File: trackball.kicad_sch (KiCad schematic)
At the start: 198 parts, among them J1 ZX-PM2.0-2-4PY, Q1 SI2302_C2891732, SW1 HX TC-5608-Y, SW2 HX TC-5608-Y, SW3 HX TC-5608-Y, SW4 HX TC-5608-Y, SW5 HX TC-5608-Y, SW6 HX TC-5608-Y, SW7 HX TC-5608-Y, SW8 HX TC-5608-Y, U1 SY8089A1AAC, U10 WS2812B, U11 WS2812B, U12 WS2812B, U13 WS2812B, U14 WS2812B, U15 WS2812B, U16 WS2812B, U17 WS2812B, U18 WS2812B, U19 WS2812B, U2 USB-TYPE-C-017, U20 WS2812B, U21 ANT3216LL00R2400A, U3 PMW3610, U4 PMW3610, U5 WS2812B, U6 WS2812B, U7 WS2812B, U8 WS2812B, U9 WS2812B, X1 XL7EL89CKI-111YLC-32M

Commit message: feat: rev.02 hardware
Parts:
- removed BAT1: ZX-SH1.0-3PLT, easyeda2kicad:CONN-SMD_3P-P1.00_HDGC_HDGC1002WV-S-3P, symbol easyeda2kicad:ZX-SH1.0-3PLT
- removed C1: CL05A106MP5NUNC_C315248, easyeda2kicad:C0402, symbol easyeda2kicad:CL05A106MP5NUNC_C315248
- removed C13, C14, C15, C17, C18, C19, C20, C24, C25, C28, C32, C33, C37, C38, C42, C46, C48, C49, C54, C55, C57: TCC0402X7R103M500AT, easyeda2kicad:C0402, symbol easyeda2kicad:TCC0402X7R103M500AT
- removed C16, C21, C22, C23, C30, C36, C43, C45, C51, C52: CC0402KRX7R7BB104, easyeda2kicad:C0402, symbol easyeda2kicad:CC0402KRX7R7BB104
- removed C2, C26, C27, C29, C4, C5, C56, C58, C59, C8: CL05A105KP5NNNC, easyeda2kicad:C0402, symbol easyeda2kicad:CL05A105KP5NNNC
- removed C3, C40, C41: CC0402FRNPO9BN120, easyeda2kicad:C0402, symbol easyeda2kicad:CC0402FRNPO9BN120
- removed C35: 0402CG1R0C500NT, easyeda2kicad:C0402, symbol easyeda2kicad:0402CG1R0C500NT
- removed C39: 0402CG1R2C500NT, easyeda2kicad:C0402, symbol easyeda2kicad:0402CG1R2C500NT
- removed C44, C50: 0402CG821J500NT, easyeda2kicad:C0402, symbol easyeda2kicad:0402CG821J500NT
- removed L1, L2: MDA4020-1R0M, easyeda2kicad:IND-SMD_L4.5-W4.1_GSSM0420, symbol easyeda2kicad:MDA4020-1R0M
- removed LED1, LED2, LED3, LED4, LED5: XL-1005UGC, easyeda2kicad:LED0402-RD_GREEN, symbol easyeda2kicad:XL-1005UGC
- removed LED15: PD15-22C/TR8, easyeda2kicad:SENSOR-SMD_PD15-22C-TR8, symbol easyeda2kicad:PD15-22C_TR8
- removed Q1: SI2302_C2891732, easyeda2kicad:SOT-23-3_L2.9-W1.3-P1.90-LS2.4-BR, symbol easyeda2kicad:SI2302_C2891732
- removed R1, R10, R15, R16, R20, R21, R22, R23, R24, R27, R28, R3, R32, R33, R34, R37, R38, R39, R4, R40, R41, R42, R45, R48, R54, R55, R68, R9: HPCR0402F160KK9, easyeda2kicad:R0402, symbol easyeda2kicad:HPCR0402F160KK9
- removed R11, R12, R13, R14, R17, R18, R19, R2, R25, R26, R29, R30, R31, R35, R36, R43, R44, R46, R47, R49, R50, R51, R56, R57, R6, R65, R66, R67, R7, R8: FRC0402F1002TS, easyeda2kicad:R0402, symbol easyeda2kicad:FRC0402F1002TS
- removed R52, R53: FRC0402P000 TS, easyeda2kicad:R0402, symbol easyeda2kicad:FRC0402P000TS
- removed SW_RST1: TS24CA, easyeda2kicad:SW-SMD_TS24CA, symbol easyeda2kicad:TS24CA
- removed U1: SY8089A1AAC, easyeda2kicad:TSOT-23-5_L2.9-W1.6-P0.95-LS2.8-BR, symbol easyeda2kicad:SY8089A1AAC
- removed U21: ANT3216LL00R2400A, easyeda2kicad:ANT-SMD_L3.2-W1.6, symbol easyeda2kicad:ANT3216LL00R2400A
- added BAT1: HCZZ0032-3, easyeda2kicad:CONN-SMD_HCZZ0032-3, symbol easyeda2kicad:HCZZ0032-3
- added C1, C14, C15, C2, C3, C51, C52, C53, C59, C62, C64, C65, C7, C72, C9: CGA0201X5R105M6R3ET, easyeda2kicad:C0201, symbol easyeda2kicad:CGA0201X5R105M6R3ET
- added C12, C16, C19, C20, C26, C27, C28, C29, C30, C31, C32, C33, C35, C39, C40, C41, C42, C43, C44, C61, C67: 0201B103K160NT, easyeda2kicad:C0201, symbol easyeda2kicad:0201B103K160NT
- added C17: GRM155R60J226ME11D, easyeda2kicad:C0402, symbol easyeda2kicad:GRM155R60J226ME11D
- added C18: CL05A106MP5NUNC_C315248, easyeda2kicad:C0402, symbol easyeda2kicad:CL05A106MP5NUNC_C315248
- added C21, C45: 0201CG120J500NT, easyeda2kicad:C0201, symbol easyeda2kicad:0201CG120J500NT
- added C22, C24, C34, C37, C47, C48, C49, C50, C54, C58: CGA0201X5R104K100ET, easyeda2kicad:C0201, symbol easyeda2kicad:CGA0201X5R104K100ET
- added C46: 0201CG1R0C250NT, easyeda2kicad:C0201, symbol easyeda2kicad:0201CG1R0C250NT
- added C57: CGA0201C0G1R2C500ET, easyeda2kicad:C0201, symbol easyeda2kicad:CGA0201C0G1R2C500ET
- added C6, C71: (no value), easyeda2kicad:C0201, symbol easyeda2kicad:CC0201KRX7R7BB151
- added C60, C63, C66: 0201B821K500NT, easyeda2kicad:C0201, symbol easyeda2kicad:0201B821K500NT
- added J1: Conn_01x02, symbol Connector_Generic:Conn_01x02
- added L1, L3: FTC252012SR47MBCA, easyeda2kicad:IND-SMD_L2.5-W2.0, symbol easyeda2kicad:FTC252012SR47MBCA
- added L2: FTC252012S1R0MBCD, easyeda2kicad:L1008, symbol easyeda2kicad:FTC252012S1R0MBCD
- added LED10, LED8: TZ-P2-0402RTIA1-0.45T, easyeda2kicad:LED0402-RD_RED, symbol easyeda2kicad:TZ-P2-0402RTIA1-0.45T
- added Q1, Q2, Q4: XR2302, easyeda2kicad:SOT-23-3_L2.9-W1.3-P0.95-LS2.4-BR, symbol easyeda2kicad:XR2302
- added R1, R10, R12, R13, R14, R15, R19, R20, R21, R29, R3, R30, R33, R34, R35, R39, R40, R43, R44, R45, R46, R47, R48, R50, R51, R52, R59, R6, R65: RC-01W103JT, easyeda2kicad:R0201, symbol easyeda2kicad:RC-01W103JT
- added R11, R16, R17, R18, R2, R22, R23, R24, R25, R26, R27, R28, R31, R32, R36, R37, R38, R41, R42, R5, R7, R8: 0201WMF1603TEE, easyeda2kicad:R0201, symbol easyeda2kicad:0201WMF1603TEE
- added R61, R63, R9: RT0402BRE0750RL, easyeda2kicad:R0402, symbol easyeda2kicad:RT0402BRE0750RL
- added SW9: TS-1010-C-A, easyeda2kicad:KEY-SMD_TX-1010-X-X, symbol easyeda2kicad:TS-1010-C-A
- added U2, U3: SY80004DQD, easyeda2kicad:VSON-6_L1.5-W1.5-P0.50-TL, symbol easyeda2kicad:SY80004DQD
- renumbered C12 to C13, C60 to C23, C47 to C25, C61 to C36, C53 to C38, C7 to C4, C6 to C5, C31 to C55, C34 to C56, C9 to C8, J1 to J2, L3 to L4, L4 to L5, LED11 to LED1, LED9 to LED11, LED8 to LED12, LED7 to LED13, LED12 to LED3, LED13 to LED4, LED6 to LED5, LED14 to LED7, LED10 to LED9, R5 to R4, R61 to R49, R62 to R53, R63 to R55, R64 to R60, R60 to R62, R59 to R64, R58 to R66, R71 to R68, U2 to U1, U9 to U10, U10 to U11, U11 to U12, U12 to U13, U13 to U14, U14 to U15, U15 to U16, U16 to U17, U17 to U18, U18 to U19, U19 to U20, U20 to U21, U3 to U4, U4 to U5, U5 to U6, U6 to U7, U7 to U8, U8 to U9
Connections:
- net 1V8: now also C2.1, C47.2, C48.2, C49.2, C50.1, C51.1, C58.2, C59.1, C6.2, C62.1, C65.1, L1.2, R10.2, R12.1, R13.2, R14.2, R16.2, R17.2, R26.2, R27.2, R31.2, R32.2, R37.2, R38.2
- net 3V3: now also C14.1, C17.1, C64.2, C71.2, C72.2, J1.2 (Pin_2), L3.2, R3.2, R52.1; no longer U_CHG1.2 (LDO)
- net ADC_BAT: now also C61.2, R50.2, R51.1
- net ADC_VBUS: now also C67.2, R18.2, R24.1
- net BAT_TS: now also BAT1.2, R47.1
- net BAT_VCC: now also BAT1.1, C7.1, R51.2
- net BCKLT_GND: now also Q4.3 (D)
- net CHG_IRQ: now also R14.1
- net CHG_ISACTIVE: no longer U_MCU1.B15 (P1.03)
- net CHG_SCL: now also R12.2
- net CHG_SDA: now also R13.1
- net D_RE1_1V8: now also R22.1, R25.2, R42.2
- net D_RE1_A: now also C44.1, R42.1
- net D_RE1_B: now also C30.2, R25.1
- net D_RE1_GND: now also C16.1, C30.1, C44.2
- net D_RE1_SW: now also C16.2, R21.1
- net D_RE2_1V8: now also R28.2, R36.1, R41.2
- net D_RE2_A: now also C43.1, R41.1
- net D_RE2_B: now also C35.2, R28.1
- net D_RE2_GND: now also C31.1, C35.1, C43.2
- net D_RE2_SW: now also C31.2, R35.1
- net D_SS1_1V8: now also C37.2, R43.2
- net D_SS1_GND: now also C37.1, C39.1, C40.1
- net D_SS1_RST: now also R43.1
- net D_SS2_1V8: now also C34.2, R44.2
- net D_SS2_GND: now also C26.1, C27.1, C34.1
- net D_SS2_RST: now also R44.1
- net GND: now also BAT1.3, BAT1.4, BAT1.5, C1.2, C12.1, C14.2, C15.2, C17.2, C18.2, C19.2, C2.2, C20.2, C21.2, C28.2, C29.2, C3.2, C32.2, C33.2, C41.2, C42.2, C45.2, C46.2, C47.1, C48.1, C49.1, C50.2, C51.2, C52.1, C53.1, C54.1, C57.1, C58.1, C59.2, C60.2, C61.1, C62.2, C63.2, C64.1, C65.2, C66.1, C67.1, C72.1, C9.2, LED10.1 (K), LED8.1 (K), Q1.2 (S), Q2.2 (S), Q4.2 (S), R11.1, R18.1, R2.1, R23.1, R45.1, R46.1, R48.1, R5.1, R50.1, R7.1, SW9.1, U2.4 (GND), U3.4 (GND); no longer U10.3 (GND), U11.3 (GND), U12.3 (GND), U13.3 (GND), U14.3 (GND), U15.3 (GND), U16.3 (GND), U17.3 (GND), U18.3 (GND), U19.3 (GND), U20.3 (GND), U21.3 (GND), U6.3 (GND), U7.3 (GND), U8.3 (GND), U9.3 (GND)
- net GNDS: now also C12.2, C9.1, R8.2
- net MCU_BCKLT_EN: now also Q4.1 (G), R46.2
- net MCU_DEC46: now also C52.2
- net MCU_LED1: now also R63.2
- net MCU_LED2: now also R61.2
- net MCU_RESET: now also C66.2, R9.2
- net MCU_XC1: now also C45.1
- net MCU_XC2: now also C21.1
- net SJ_NOTS1: now also R47.2
- net SW1: now also C20.1, R19.2
- net SW2: now also C19.1, R20.2
- net SW3: now also C28.1, R30.2
- net SW4: now also C29.1, R29.2
- net SW5: now also C41.1, R33.2
- net SW6: now also C32.1, R34.2
- net SW7: now also C42.1, R40.2
- net SW8: now also C33.1, R39.2
- net USB_MUX_SEL: now also R11.2
- net USB_VBUS: now also J2.8, C1.1, C53.2, R24.2
- net VSYS: now also C15.1, C18.1, C3.1, L2.2, R1.1, R15.2, R59.1, R65.2, U2.6 (IN), U3.6 (IN)
- net at SW7.1: now also R17.1, R40.1
- net at L4.1, L5.2: now also C57.2
- net at U_MCU1.C1 (DEC1): now also C54.2
- net at U5.1 (+VCSEL), U5.10 (PASS_T): now also C27.2
- net at SW5.1: now also R26.1, R33.1
- net at SW4.1: now also R29.1, R31.1
- net at C38.2, U5.9 (VCP): now also C26.2
- net at SW1.1: now also R19.1, R37.1
- net at U4.1 (+VCSEL), U4.10 (PASS_T): now also C40.2
- net at U4.12 (CP): now also C22.2
- net at U4.13 (CN): now also C22.1
- net at C25.2, U4.9 (VCP): now also C39.2
- net at C11.2, R4.2, U_CHG1.10 (BAT)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: now also C7.2
- net at U_MCU1.D23 (DEC3): now also C60.1
- net at SW3.1: now also R30.1, R32.1
- net at U5.12 (CP): now also C24.2
- net at U5.13 (CN): now also C24.1
- net at SW8.1: now also R16.1, R39.1
- net at U_MUX1.8 (~{OE}): now also R2.2
- net at SW2.1: now also R20.1, R38.1
- net at U_RE2.E: now also R35.2, R36.2
- net at U_RE1.E: now also R21.2, R22.2
- net at L5.1, U_MCU1.H23 (ANT): now also C46.1
- net at U_MCU1.N24 (DEC5): now also C63.1
- net at LED5.2 (A): now also R52.2
- net at SW6.1: now also R27.1, R34.1
- net at U_CHG1.15 (SW), U_CHG1.16 (SW), U_CHG1.17 (SW)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: now also L2.1
- net CHG_ADC: no longer names the net of U_CHG1.6 (GPADC)
- net MCU_LED3 renamed MCU_VIB_EN
- net MCU_VIB_EN: now also Q2.1 (G), R48.2
- new net: R7.2, R8.1
- new net: R1.2, U3.1 (EN)
- new net: R15.1, U3.2 (PG)
- new net: R9.1, SW9.2
- new net: C6.1, R10.1, R5.2, U2.3 (FB)
- new net: R3.1, R6.2
- new net: LED10.2 (A), R63.1
- new net: R59.2, U2.1 (EN)
- new net: C71.1, R23.2, R6.1, U3.3 (FB)
- new net: R65.1, U2.2 (PG)
- new net: L1.1, U2.5 (LX)
- new net: LED8.2 (A), R61.1
- new net: L3.1, U3.5 (LX)
- new net MCU_RGB_EN: Q1.1 (G), R45.2, U_MCU1.B15 (P1.03)
- new net RGB_GND: Q1.3 (D), U10.3 (GND), U11.3 (GND), U12.3 (GND), U13.3 (GND), U14.3 (GND), U15.3 (GND), U16.3 (GND), U17.3 (GND), U18.3 (GND), U19.3 (GND), U20.3 (GND), U21.3 (GND), U6.3 (GND), U7.3 (GND), U8.3 (GND), U9.3 (GND)
- new net VIB_GND: J1.1 (Pin_1), Q2.3 (D)
- no-connect marks 54 -> 51
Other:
- note added: "3.3V"
- note added: "actually 3.15V"
- note added: "actually ~1.875V for LEDs stability and to ensure no need in voltage level converter"
- note removed: "alternative antenna? 5dBi stated"
- note removed: "in case if mux isn't populated"
- note removed: "programming/debug port"
- moved on the sheet: AE1, C10, C11, C13, C23, C25, C36, C38, C4, C5, C55, C56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

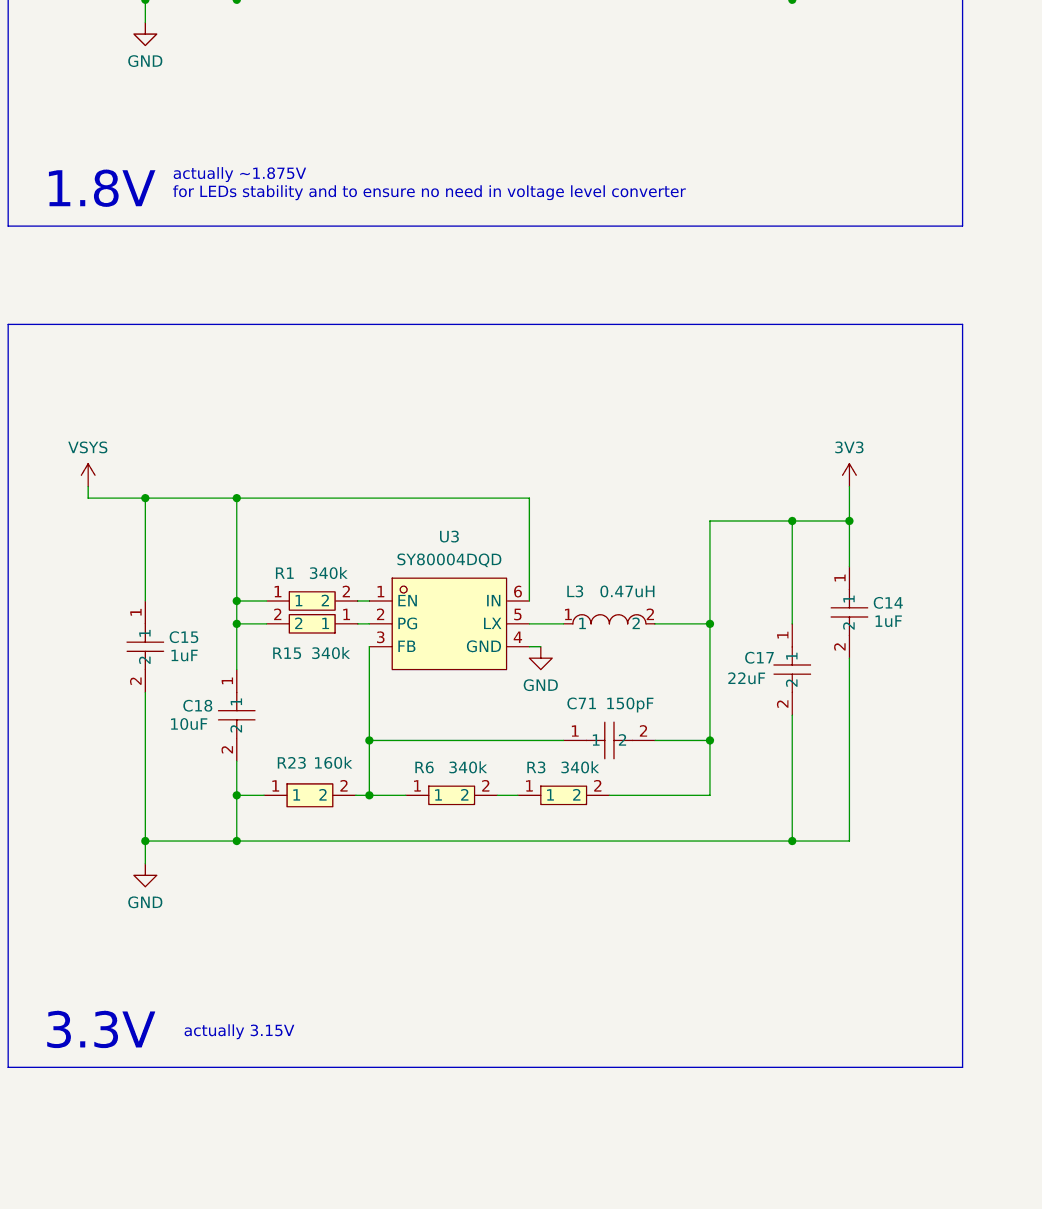
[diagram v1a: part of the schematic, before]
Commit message: chore: refactoring
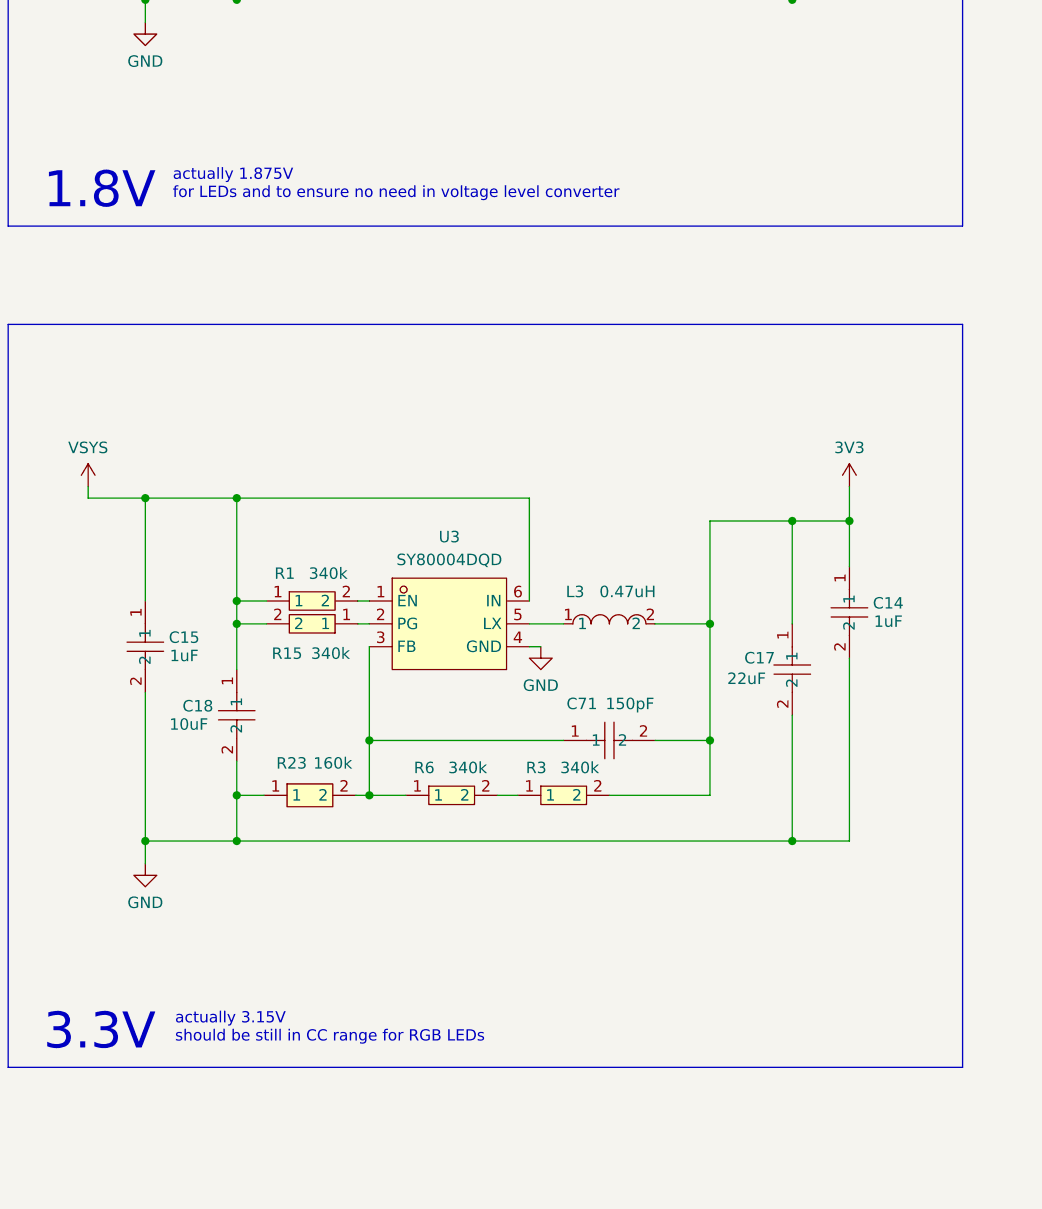
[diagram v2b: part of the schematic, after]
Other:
- note added: "actually 1.875V for LEDs and to ensure no need in voltage level converter"
- note added: "actually 3.15V should be still in CC range for RGB LEDs"
- note removed: "actually 3.15V"
- note removed: "actually ~1.875V for LEDs stability and to ensure no need in voltage level converter"
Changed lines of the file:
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@@
 		)
 	)
-	(text "actually 3.15V"
+	(text "actually 3.15V\nshould be still in CC range for RGB LEDs"
 		(exclude_from_sim no)
-		(at 475.742 193.802 0)
+		(at 468.63 193.294 0)
 		(effects
 			(font
@@
 				(color 168 168 168 1)
 			)
+			(justify left)
 		)
 	)
-	(text "actually ~1.875V \nfor LEDs stability and to ensure no need in voltage level converter"
+	(text "actually 1.875V \nfor LEDs and to ensure no need in voltage level converter"
 		(exclude_from_sim no)
 		(at 468.376 99.568 0)

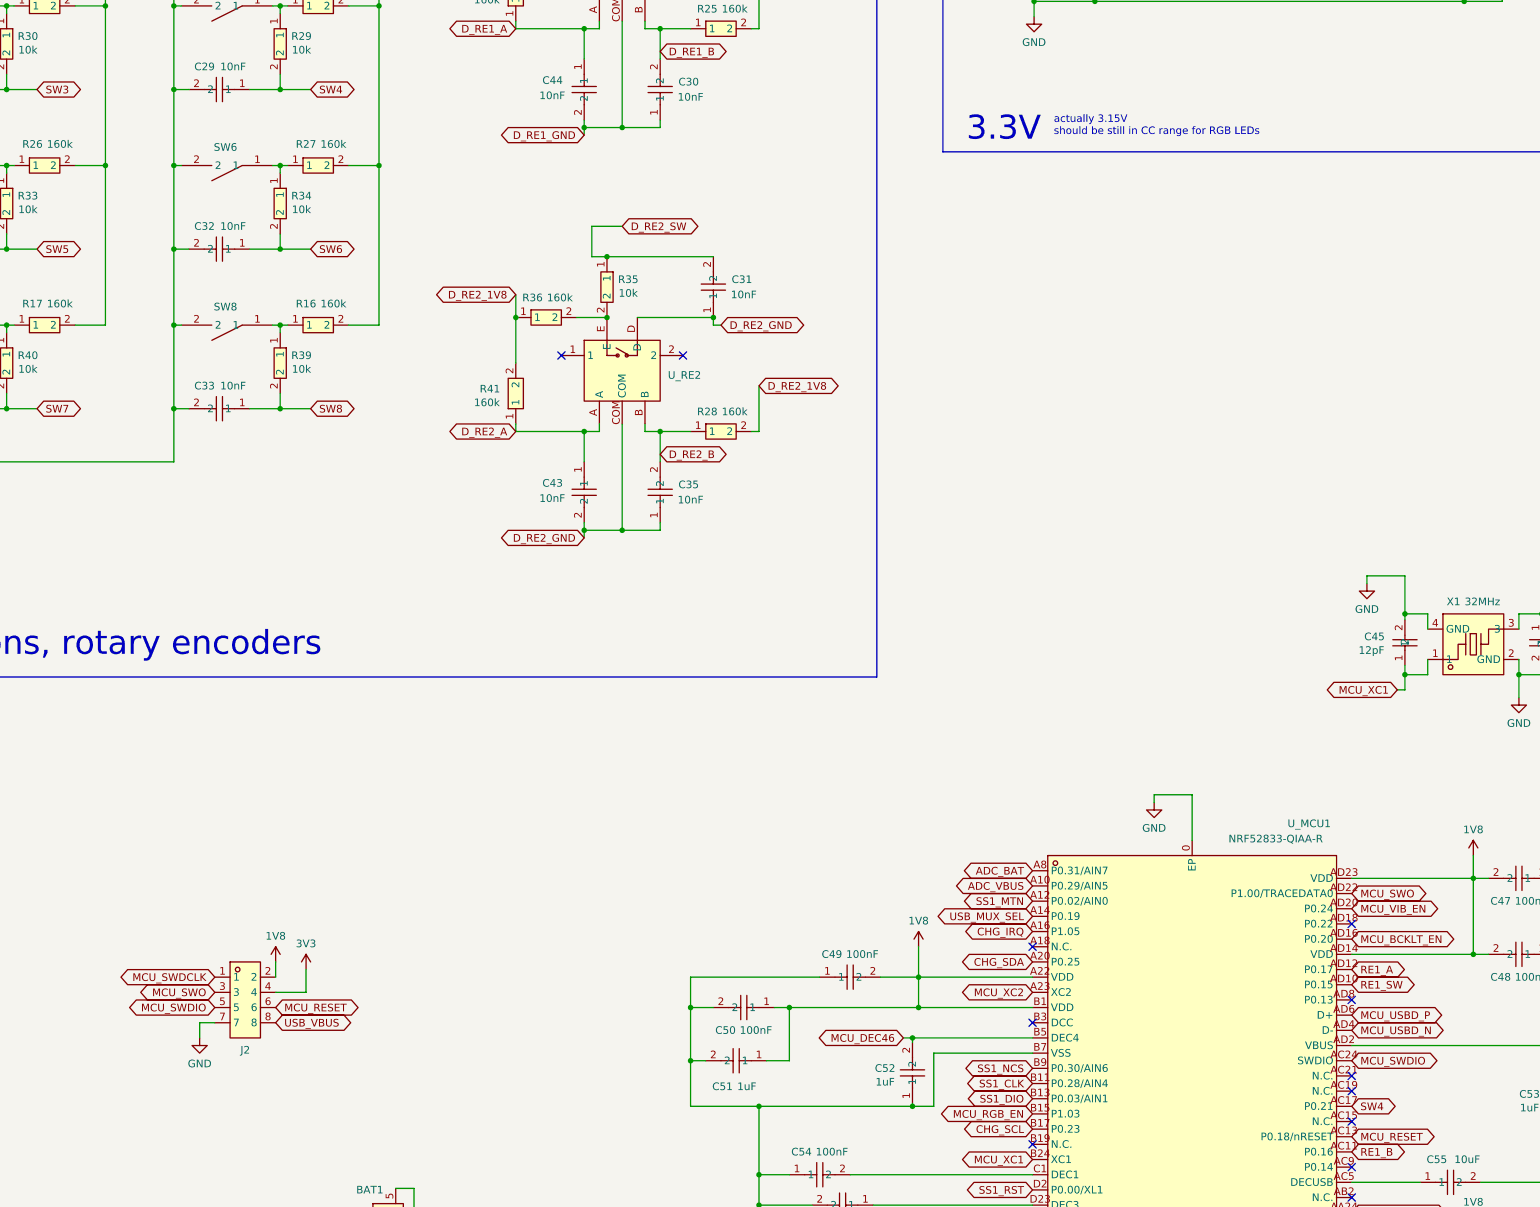
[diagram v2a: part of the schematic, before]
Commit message: chore: refactoring
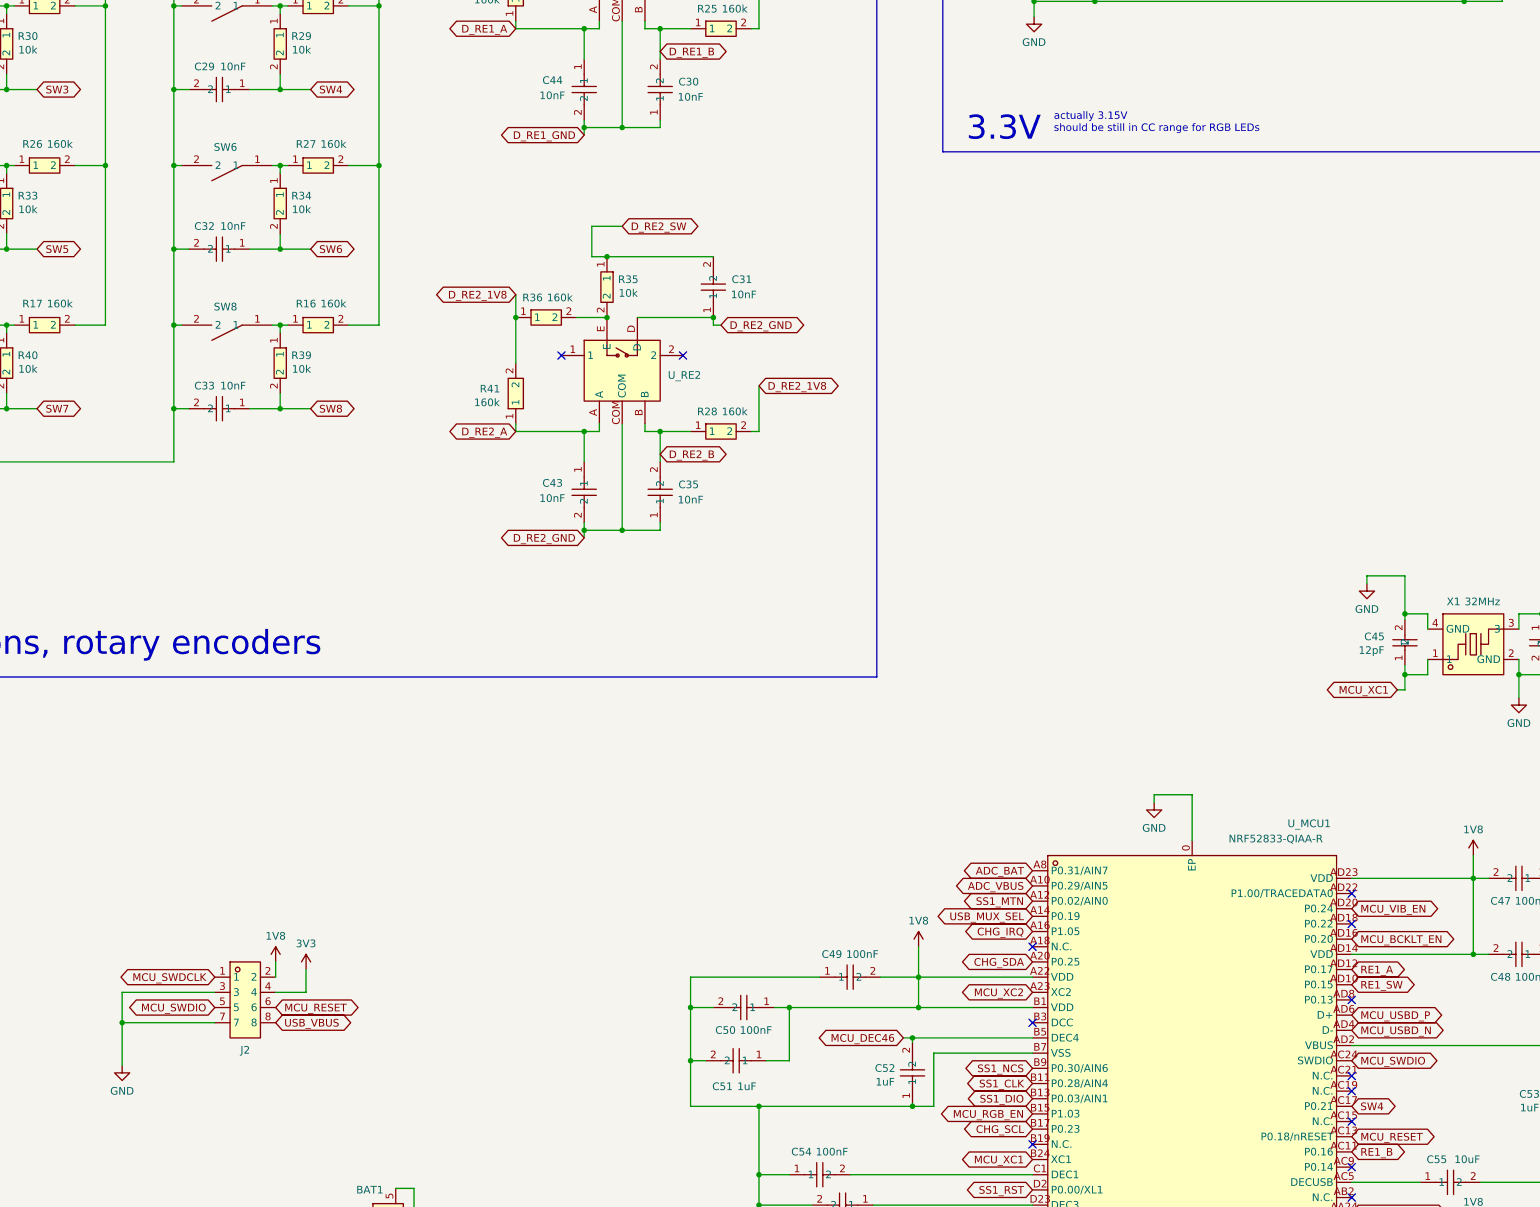
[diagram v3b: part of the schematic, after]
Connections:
- net GND: now also J2.3
- net MCU_SWO: no longer names the net of U_MCU1.AD22 (P1.00/TRACEDATA0)
- net MCU_SWO: no longer J2.3
- no-connect marks 51 -> 52
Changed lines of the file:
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@@
 	(text "actually 3.15V\nshould be still in CC range for RGB LEDs"
 		(exclude_from_sim no)
-		(at 468.63 193.294 0)
+		(at 468.63 192.786 0)
 		(effects
 			(font
@@
 	)
 	(junction
+		(at 312.928 343.154)
+		(diameter 0)
+		(color 0 0 0 0)
+	)
+	(junction
 		(at 475.488 40.894)
 		(diameter 0)
@@
 	)
 	(no_connect
+		(at 518.414 321.564)
+	)
+	(no_connect
 		(at 386.334 231.648)
 	)
@@
 	(wire
 		(pts
+			(xy 312.928 338.074) (xy 312.928 343.154)
+		)
+		(stroke
+			(width 0)
+			(type default)
+		)
+	)
+	(wire
+		(pts
 			(xy 221.488 165.1) (xy 221.488 171.45)
 		)
@@
 	(wire
 		(pts
-			(xy 325.882 343.154) (xy 328.422 343.154)
+			(xy 312.928 343.154) (xy 328.422 343.154)
 		)
 		(stroke
@@
 	(wire
 		(pts
+			(xy 312.928 338.074) (xy 328.422 338.074)
+		)
+		(stroke
+			(width 0)
+			(type default)
+		)
+	)
+	(wire
+		(pts
 			(xy 390.144 259.588) (xy 390.144 260.858)
 		)
@@
 	(wire
 		(pts
-			(xy 325.882 343.154) (xy 325.882 345.694)
+			(xy 312.928 343.154) (xy 312.928 350.266)
 		)
 		(stroke
@@
 		)
 	)
-	(global_label "MCU_SWO"
-		(shape bidirectional)
-		(at 328.422 338.074 180)
-		(fields_autoplaced yes)
-		(effects
-			(font
-				(size 1.27 1.27)
-			)
-			(justify right)
-		)
-		(property "Intersheetrefs" "${INTERSHEET_REFS}"
-			(at 315.3146 338.074 0)
-			(effects
-				(font
-					(size 1.27 1.27)
-				)
-				(justify right)
-				(hide yes)
-			)
-		)
-	)
 	(global_label "D_SS2_GND"
 		(shape bidirectional)
@@
 		)
 	)
-	(global_label "MCU_SWO"
-		(shape bidirectional)
-		(at 518.414 321.564 0)
-		(fields_autoplaced yes)
-		(effects
-			(font
-				(size 1.27 1.27)
-			)
-			(justify left)
-		)
-		(property "Intersheetrefs" "${INTERSHEET_REFS}"
-			(at 531.5214 321.564 0)
-			(effects
-				(font
-					(size 1.27 1.27)
-				)
-				(justify left)
-				(hide yes)
-			)
-		)
-	)
 	(global_label "SW5"
 		(shape bidirectional)
@@
 	(symbol
 		(lib_id "power:GND")
-		(at 325.882 345.694 0)
+		(at 312.928 350.266 0)
 		(unit 1)
 		(exclude_from_sim no)
@@
 		(dnp no)
 		(property "Reference" "#PWR044"
-			(at 325.882 352.044 0)
+			(at 312.928 356.616 0)
 			(effects
 				(font
@@
 		)
 		(property "Value" "GND"
-			(at 325.882 350.012 0)
+			(at 312.928 354.584 0)
 			(effects
 				(font
@@
 		)
 		(property "Footprint" ""
-			(at 325.882 345.694 0)
+			(at 312.928 350.266 0)
 			(effects
 				(font
@@
 		)
 		(property "Datasheet" ""
-			(at 325.882 345.694 0)
+			(at 312.928 350.266 0)
 			(effects
 				(font
@@
 		)
 		(property "Description" "Power symbol creates a global label with name \"GND\" , ground"
-			(at 325.882 345.694 0)
+			(at 312.928 350.266 0)
 			(effects
 				(font
